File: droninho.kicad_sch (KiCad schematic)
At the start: 28 parts, among them J1 Conn_01x06_Socket, J2 Conn_01x02_Socket, J3 Conn_01x02_Socket, J4 Conn_01x02_Socket, J5 Conn_01x02_Socket, Q1 Si2300DS, Q2 Si2300DS, Q3 Si2300DS, Q4 Si2300DS, U1 AMS1117-3.3

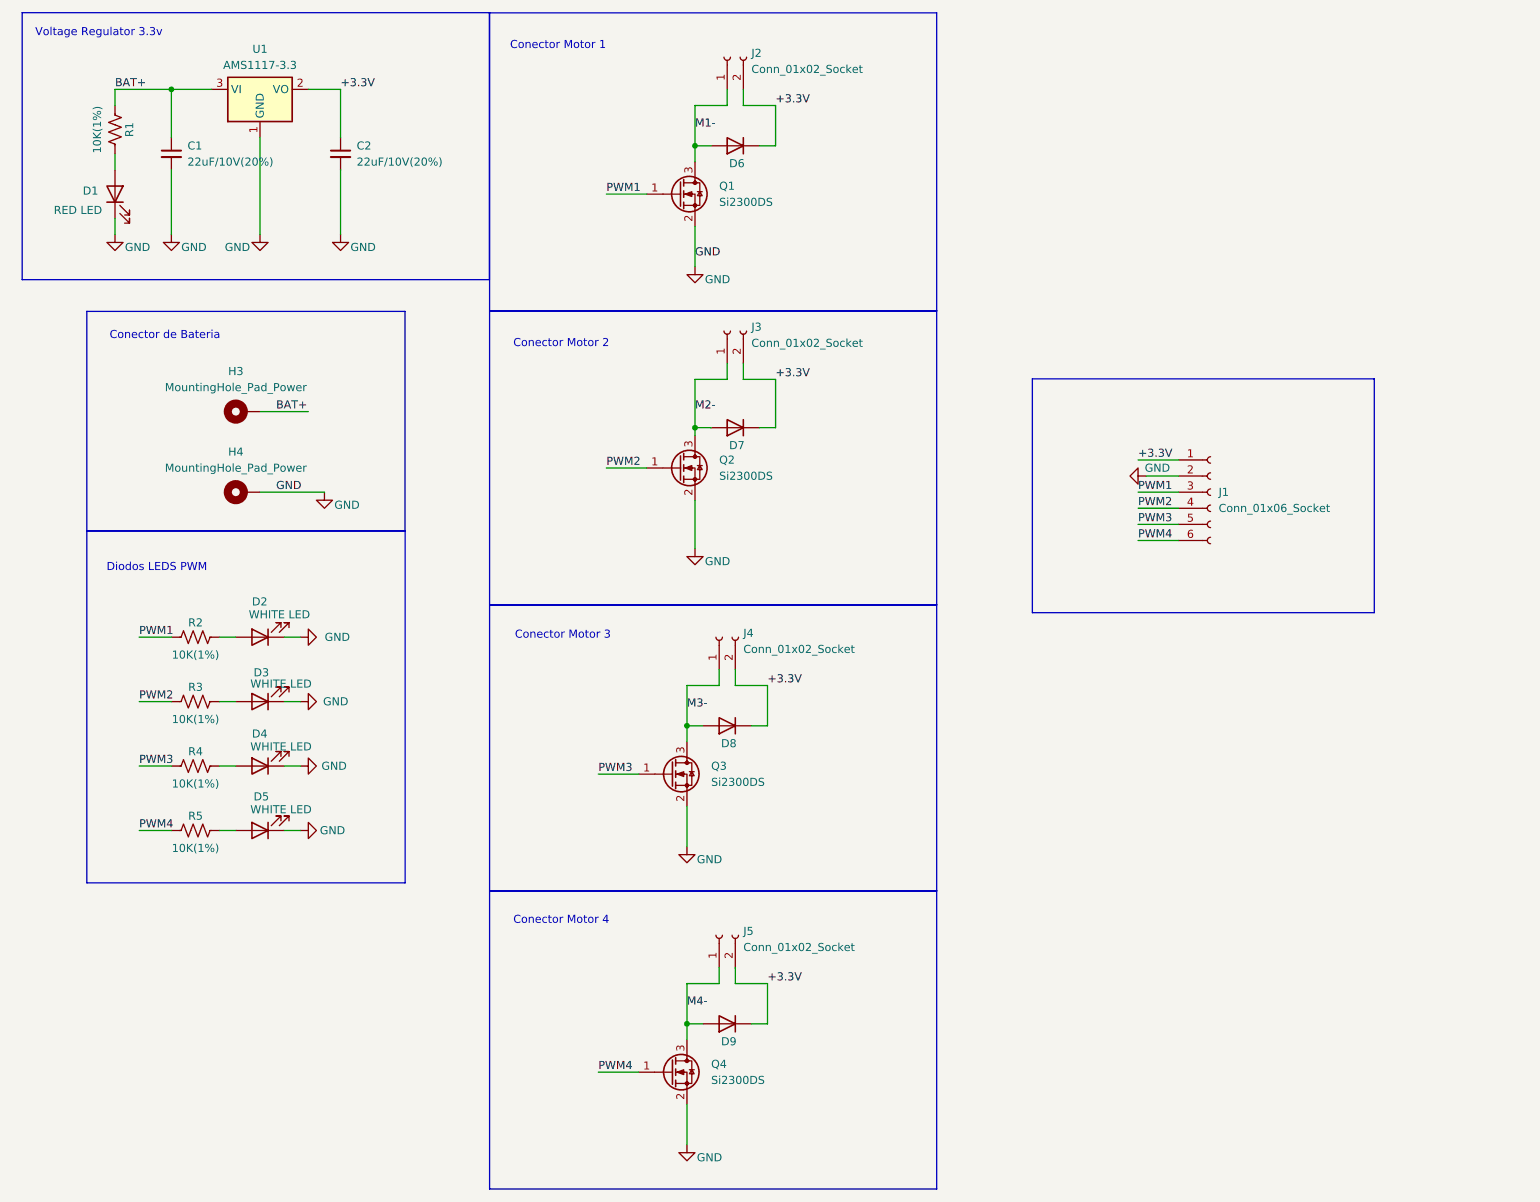
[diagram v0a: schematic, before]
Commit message: small updates
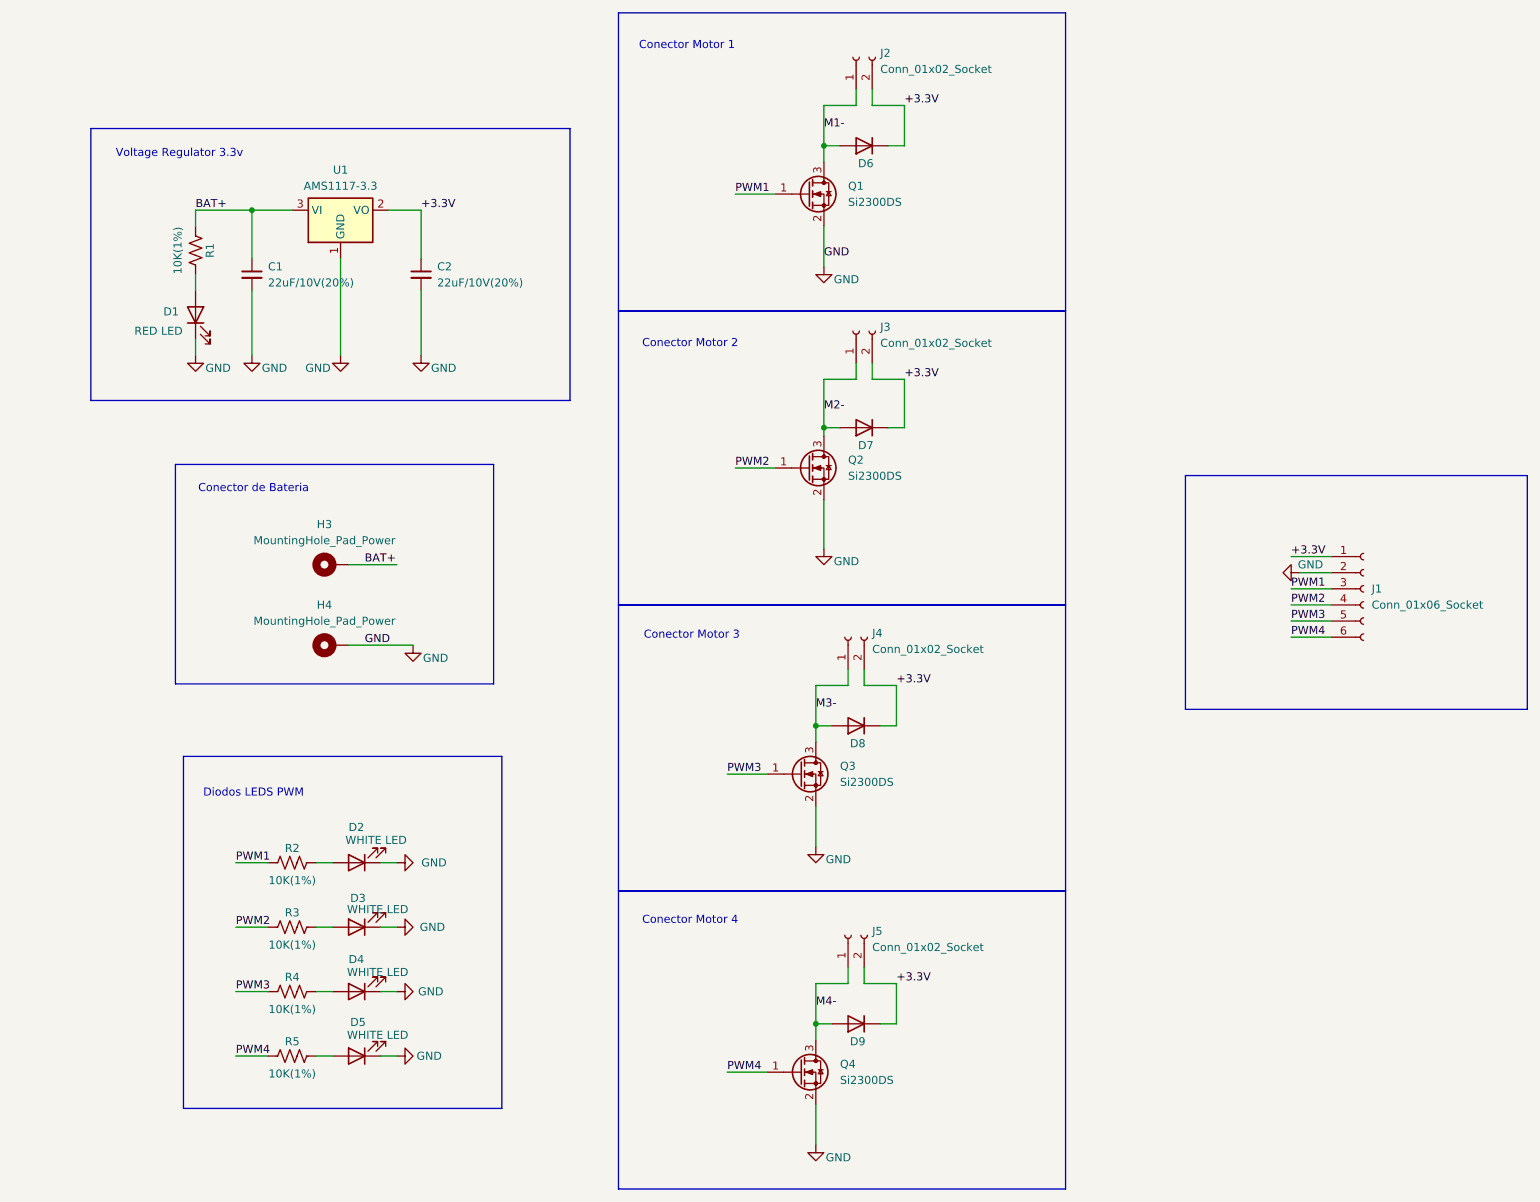
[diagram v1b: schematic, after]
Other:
- moved on the sheet: C1, C2, D1, D2, D3, D4, D5, D6, D7, D8, D9, H3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

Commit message: driver finalizado.
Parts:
- J1: footprint Connector_Hirose:Hirose_DF13-06P-1.25DSA_1x06_P1.25mm_Vertical -> Connector_JST:JST_PH_B6B-PH-K_1x06_P2.00mm_Vertical; Designator (none) -> J1; Manufacturer (none) -> JST Commercial; Mfg Part # (none) -> BM06B-PASS-TF(LF)(SN); Package/Footprint (none) -> 6POS; Type (none) -> thru-hole
- J2: footprint Connector_Hirose:Hirose_DF13-02P-1.25DSA_1x02_P1.25mm_Vertical -> Connector_JST:JST_PH_B2B-PH-K_1x02_P2.00mm_Vertical; Designator (none) -> J2; Manufacturer (none) -> JST Commercial; Mfg Part # (none) -> BM02B-PASS-TF(LF)(SN); Package/Footprint (none) -> 2POS; Type (none) -> thru-hole
- J3: footprint Connector_Hirose:Hirose_DF13-02P-1.25DSA_1x02_P1.25mm_Vertical -> Connector_JST:JST_PH_B2B-PH-K_1x02_P2.00mm_Vertical; Designator (none) -> J3; Manufacturer (none) -> JST Commercial; Mfg Part # (none) -> BM02B-PASS-TF(LF)(SN); Package/Footprint (none) -> 2POS; Type (none) -> thru-hole
- J4: footprint Connector_Hirose:Hirose_DF13-02P-1.25DSA_1x02_P1.25mm_Vertical -> Connector_JST:JST_PH_B2B-PH-K_1x02_P2.00mm_Vertical; Designator (none) -> J4; Manufacturer (none) -> JST Commercial; Mfg Part # (none) -> BM02B-PASS-TF(LF)(SN); Package/Footprint (none) -> 2POS; Type (none) -> thru-hole
- J5: footprint Connector_Hirose:Hirose_DF13-02P-1.25DSA_1x02_P1.25mm_Vertical -> Connector_JST:JST_PH_B2B-PH-K_1x02_P2.00mm_Vertical; Designator (none) -> J5; Manufacturer (none) -> JST Commercial; Mfg Part # (none) -> BM02B-PASS-TF(LF)(SN); Package/Footprint (none) -> 2POS; Type (none) -> thru-hole
- U1: Designator (none) -> U1; Manufacturer (none) -> Texas Instruments; Mfg Part # (none) -> LM1117MPX-3.3/NOPB; Package/Footprint (none) -> SOT-223-4; Type (none) -> SMD
